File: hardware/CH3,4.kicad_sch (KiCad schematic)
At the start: 104 parts, among them J2 RJ45, J3 RJ45, U10 ADG719, U11 INA828, U12 OPA2192, U13 OPA2192, U14 INA828, U15 SGM2059, U4 INA828, U5 OPA2192, U6 OPA2192, U7 INA828, U8 SGM2059, U9 ADG719

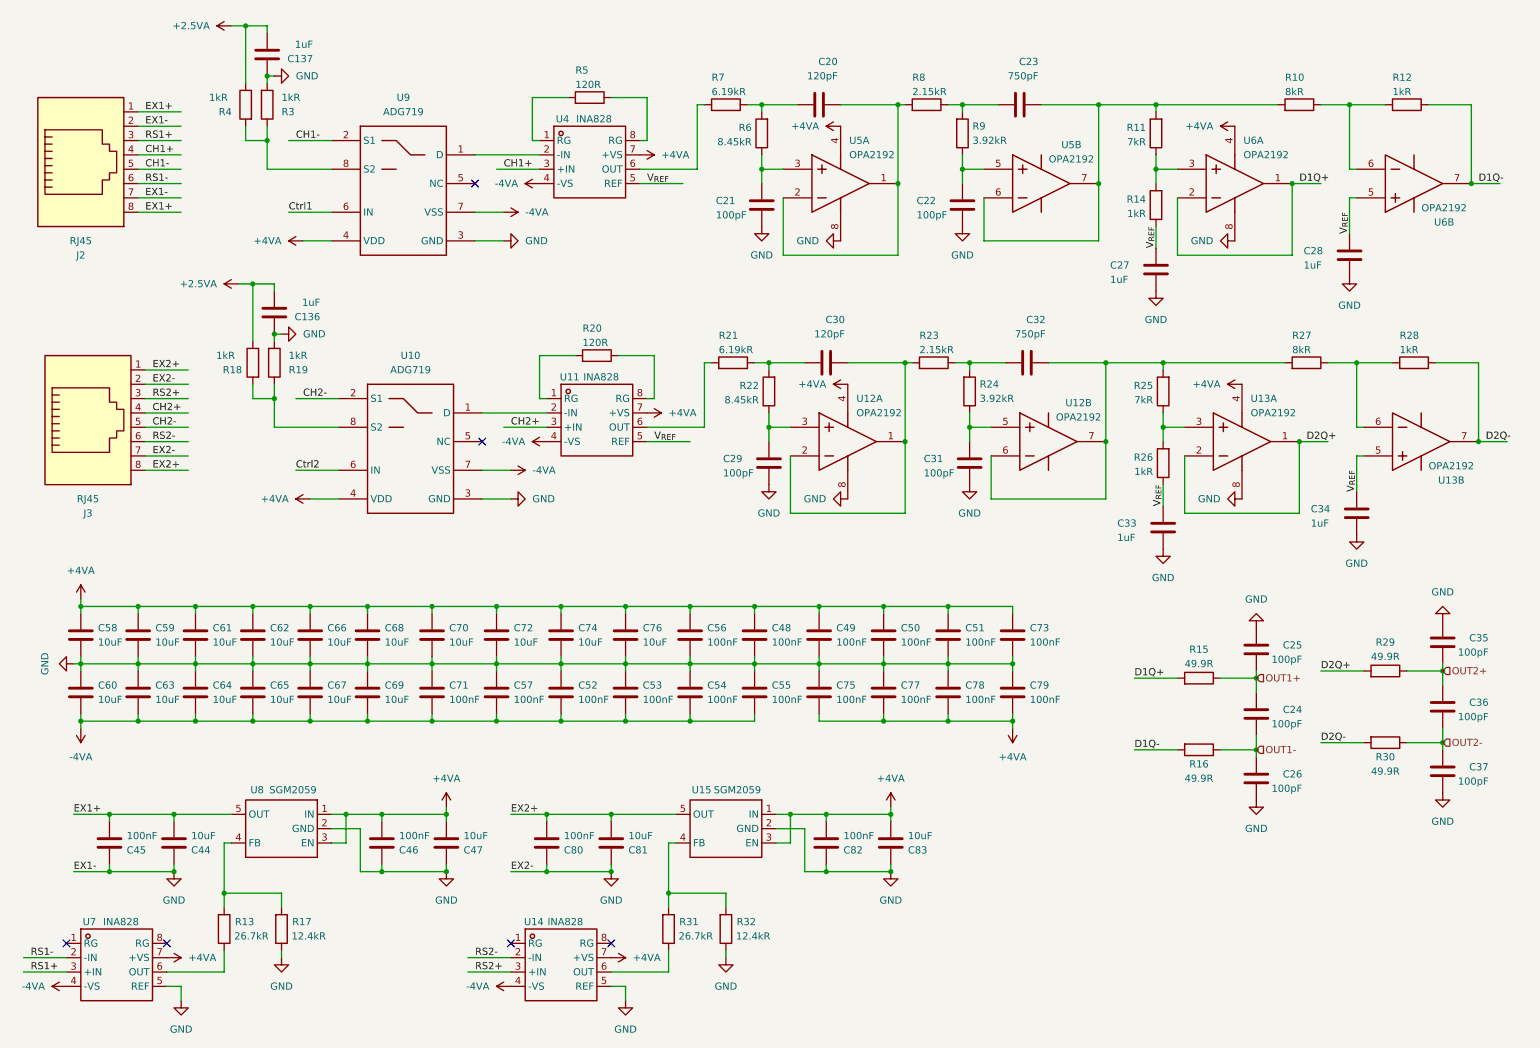
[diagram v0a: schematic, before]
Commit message: feat：远程感测原理图；多路通道
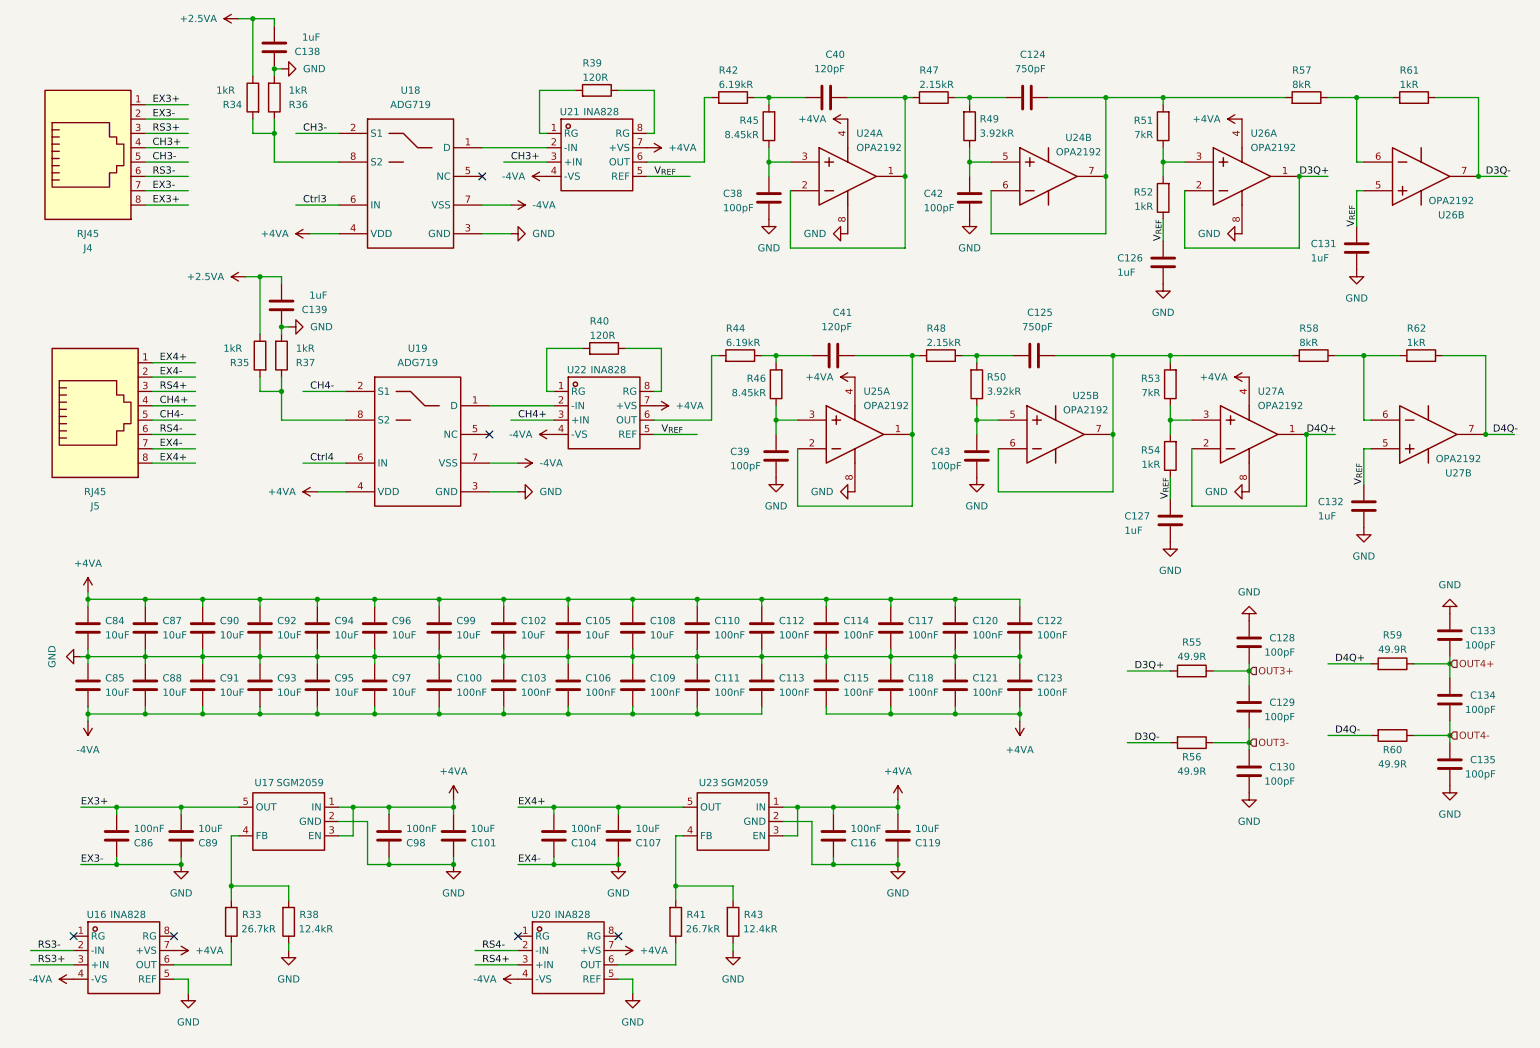
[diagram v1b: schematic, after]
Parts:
- removed C136, C137, C27, C28, C33, C34: 1uF, Capacitor_SMD:C_0603_1608Metric, symbol Device:C
- removed C20, C30: 120pF, Capacitor_SMD:C_0603_1608Metric, symbol Device:C
- removed C21, C22, C24, C25, C26, C29, C31, C35, C36, C37: 100pF, Capacitor_SMD:C_0603_1608Metric, symbol Device:C
- removed C23, C32: 750pF, Capacitor_SMD:C_0603_1608Metric, symbol Device:C
- removed C44, C47, C58, C59, C60, C61, C62, C63, C64, C65, C66, C67, C68, C69, C70, C72, C74, C76, C81, C83: 10uF, Capacitor_SMD:C_0603_1608Metric, symbol Device:C
- removed C45, C46, C48, C49, C50, C51, C52, C53, C54, C55, C56, C57, C71, C73, C75, C77, C78, C79, C80, C82: 100nF, Capacitor_SMD:C_0603_1608Metric, symbol Device:C
- removed J2, J3: RJ45, Connector_RJ:RJ45_Amphenol_54602-x08_Horizontal, symbol Connector:RJ45
- removed R10, R27: 8kR, Resistor_SMD:R_0603_1608Metric, symbol Device:R
- removed R11, R25: 7kR, Resistor_SMD:R_0603_1608Metric, symbol Device:R
- removed R12, R14, R18, R19, R26, R28, R3, R4: 1kR, Resistor_SMD:R_0603_1608Metric, symbol Device:R
- removed R13, R31: 26.7kR, Resistor_SMD:R_0603_1608Metric, symbol Device:R
- removed R15, R16, R29, R30: 49.9R, Resistor_SMD:R_0603_1608Metric, symbol Device:R
- removed R17, R32: 12.4kR, Resistor_SMD:R_0603_1608Metric, symbol Device:R
- removed R20, R5: 120R, Resistor_SMD:R_0603_1608Metric, symbol Device:R
- removed R21, R7: 6.19kR, Resistor_SMD:R_0603_1608Metric, symbol Device:R
- removed R22, R6: 8.45kR, Resistor_SMD:R_0603_1608Metric, symbol Device:R
- removed R23, R8: 2.15kR, Resistor_SMD:R_0603_1608Metric, symbol Device:R
- removed R24, R9: 3.92kR, Resistor_SMD:R_0603_1608Metric, symbol Device:R
- removed U10, U9: ADG719, ProPrj_New Project_2026-05-28_15-29-15_2026-05-30:SOT-23-8_L3.0-W1.7-P0.65-LS2.8-TL, symbol Analog_Switch:ADG619BRTZ-REEL7
- removed U11, U14, U4, U7: INA828, Package_SO:Infineon_PG-DSO-8-43, symbol Amplifier_Instrumentation:INA828IDR
- removed U12, U13, U5, U6: OPA2192, Package_SO:SOIC-8_3.9x4.9mm_P1.27mm, symbol Amplifier_Operational:OPA2192IDR
- removed U15, U8: SGM2059, Package_TO_SOT_SMD:SOT-23-5, symbol Regulator_Linear:SGM2059-ADJXN5G/TR
- added C100, C103, C104, C106, C109, C110, C111, C112, C113, C114, C115, C116, C117, C118, C120, C121, C122, C123, C86, C98: 100nF, Capacitor_SMD:C_0603_1608Metric, symbol Device:C
- added C101, C102, C105, C107, C108, C119, C84, C85, C87, C88, C89, C90, C91, C92, C93, C94, C95, C96, C97, C99: 10uF, Capacitor_SMD:C_0603_1608Metric, symbol Device:C
- added C124, C125: 750pF, Capacitor_SMD:C_0603_1608Metric, symbol Device:C
- added C126, C127, C131, C132, C138, C139: 1uF, Capacitor_SMD:C_0603_1608Metric, symbol Device:C
- added C128, C129, C130, C133, C134, C135, C38, C39, C42, C43: 100pF, Capacitor_SMD:C_0603_1608Metric, symbol Device:C
- added C40, C41: 120pF, Capacitor_SMD:C_0603_1608Metric, symbol Device:C
- added J4, J5: RJ45, Connector_RJ:RJ45_Amphenol_54602-x08_Horizontal, symbol Connector:RJ45
- added R33, R41: 26.7kR, Resistor_SMD:R_0603_1608Metric, symbol Device:R
- added R34, R35, R36, R37, R52, R54, R61, R62: 1kR, Resistor_SMD:R_0603_1608Metric, symbol Device:R
- added R38, R43: 12.4kR, Resistor_SMD:R_0603_1608Metric, symbol Device:R
- added R39, R40: 120R, Resistor_SMD:R_0603_1608Metric, symbol Device:R
- added R42, R44: 6.19kR, Resistor_SMD:R_0603_1608Metric, symbol Device:R
- added R45, R46: 8.45kR, Resistor_SMD:R_0603_1608Metric, symbol Device:R
- added R47, R48: 2.15kR, Resistor_SMD:R_0603_1608Metric, symbol Device:R
- added R49, R50: 3.92kR, Resistor_SMD:R_0603_1608Metric, symbol Device:R
- added R51, R53: 7kR, Resistor_SMD:R_0603_1608Metric, symbol Device:R
- added R55, R56, R59, R60: 49.9R, Resistor_SMD:R_0603_1608Metric, symbol Device:R
- added R57, R58: 8kR, Resistor_SMD:R_0603_1608Metric, symbol Device:R
- added U16, U20, U21, U22: INA828, Package_SO:Infineon_PG-DSO-8-43, symbol Amplifier_Instrumentation:INA828IDR
- added U17, U23: SGM2059, Package_TO_SOT_SMD:SOT-23-5, symbol Regulator_Linear:SGM2059-ADJXN5G/TR
- added U18, U19: ADG719, ProPrj_New Project_2026-05-28_15-29-15_2026-05-30:SOT-23-8_L3.0-W1.7-P0.65-LS2.8-TL, symbol Analog_Switch:ADG619BRTZ-REEL7
- added U24, U25, U26, U27: OPA2192, Package_SO:SOIC-8_3.9x4.9mm_P1.27mm, symbol Amplifier_Operational:OPA2192IDR
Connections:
- net +2.5VA: now also C138.2, C139.2, R34.1, R35.1
- net +4VA: now also C101.2, C102.1, C105.1, C108.1, C110.2, C112.2, C114.2, C115.1, C116.2, C117.2, C118.1, C119.2, C120.2, C121.1, C122.2, C123.1, C84.1, C87.1, C90.1, C92.1, C94.1, C96.1, C98.2, C99.1, U16.7 (+VS), U17.1 (IN), U17.3 (EN), U18.4 (VDD), U19.4 (VDD), U20.7 (+VS), U21.7 (+VS), U22.7 (+VS), U23.1 (IN), U23.3 (EN), U24.4 (VSS), U25.4 (VSS), U26.4 (VSS), U27.4 (VSS)
- net -4VA: now also C100.1, C103.1, C106.1, C109.1, C111.1, C113.1, C85.2, C88.2, C91.2, C93.2, C95.2, C97.2, U16.4 (-VS), U18.7 (VSS), U19.7 (VSS), U20.4 (-VS), U21.4 (-VS), U22.4 (-VS)
- net GND: now also C100.2, C101.1, C102.2, C103.2, C104.1, C105.2, C106.2, C107.1, C108.2, C109.2, C110.1, C111.2, C112.1, C113.2, C114.1, C115.2, C116.1, C117.1, C118.2, C119.1, C120.1, C121.2, C122.1, C123.2, C126.2, C127.2, C128.1, C130.2, C131.2, C132.2, C133.1, C135.2, C138.1, C139.1, C38.2, C39.2, C42.2, C43.2, C84.2, C85.1, C86.1, C87.2, C88.1, C89.1, C90.2, C91.1, C92.2, C93.1, C94.2, C95.1, C96.2, C97.1, C98.1, C99.2, J4.2, J4.7, J5.2, J5.7, R36.2, R37.2, R38.1, R43.1, U16.5 (REF), U17.2 (GND), U18.3 (GND), U19.3 (GND), U20.5 (REF), U23.2 (GND), U24.8 (VDD), U25.8 (VDD), U26.8 (VDD), U27.8 (VDD)
- net V_{REF}: now also C126.1, C127.1, C131.1, C132.1, R52.1, R54.1, U21.5 (REF), U22.5 (REF), U26.5 (VINB+), U27.5 (VINB+)
- new net: C40.2, R42.1, R45.2
- new net: R42.2, U21.6 (OUT)
- new net: R33.1, U16.6 (OUT)
- new net: R39.2, U21.1 (RG)
- new net: U18.1 (D), U21.2 (-IN)
- new net: R39.1, U21.8 (RG)
- new net: R58.1, R62.2, U27.6 (VINB-)
- new net: C38.1, R45.1, U24.3 (VINA+)
- new net: R40.2, U22.1 (RG)
- new net: U19.1 (D), U22.2 (-IN)
- new net: R44.2, U22.6 (OUT)
- new net: R40.1, U22.8 (RG)
- new net: R34.2, R36.1, U18.8 (S2)
- new net: C43.1, R50.1, U25.5 (VINB+)
- new net: C125.1, R53.2, R58.2, U25.6 (VINB-), U25.7 (VOUTB)
- new net: R57.1, R61.2, U26.6 (VINB-)
- new net: C124.1, R51.2, R57.2, U24.6 (VINB-), U24.7 (VOUTB)
- new net: C42.1, R49.1, U24.5 (VINB+)
- new net: R51.1, R52.2, U26.3 (VINA+)
- new net: R41.1, U20.6 (OUT)
- new net: R41.2, R43.2, U23.4 (FB)
- new net: R53.1, R54.2, U27.3 (VINA+)
- new net: C125.2, R48.1, R50.2
- new net: C39.1, R46.1, U25.3 (VINA+)
- new net: C41.2, R44.1, R46.2
- new net: C124.2, R47.1, R49.2
- new net: C41.1, R48.2, U25.1 (VOUTA), U25.2 (VINA-)
- new net: C40.1, R47.2, U24.1 (VOUTA), U24.2 (VINA-)
- new net: R33.2, R38.2, U17.4 (FB)
- new net: R35.2, R37.1, U19.8 (S2)
- new net CH3+: J4.4, U21.3 (+IN)
- new net CH3-: J4.5, U18.2 (S1)
- new net CH4+: J5.4, U22.3 (+IN)
- new net CH4-: J5.5, U19.2 (S1)
- new net Ctrl3: U18.6 (IN)
- new net Ctrl4: U19.6 (IN)
- new net D3Q+: R55.2, U26.1 (VOUTA), U26.2 (VINA-)
- new net D3Q-: R56.2, R61.1, U26.7 (VOUTB)
- new net D4Q+: R59.2, U27.1 (VOUTA), U27.2 (VINA-)
- new net D4Q-: R60.2, R62.1, U27.7 (VOUTB)
- new net EX3+: C86.2, C89.2, J4.1, J4.8, U17.5 (OUT)
- new net EX4+: C104.2, C107.2, J5.1, J5.8, U23.5 (OUT)
- new net OUT3+: C128.2, C129.1, R55.1
- new net OUT3-: C129.2, C130.1, R56.1
- new net OUT4+: C133.2, C134.1, R59.1
- new net OUT4-: C134.2, C135.1, R60.1
- new net RS3+: J4.3, U16.3 (+IN)
- new net RS3-: J4.6, U16.2 (-IN)
- new net RS4+: J5.3, U20.3 (+IN)
- new net RS4-: J5.6, U20.2 (-IN)
